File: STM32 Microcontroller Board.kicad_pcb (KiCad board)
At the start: 4 copper layers, 69.1 x 94.3 mm, 177 parts, among them J1 F407 SWD, J10 USB_B_Micro, J2 GPIO, J3 Conn_01x02_Pin, J4 F103 SWD, J5 USB_B_Micro, J6 Ethernet, J7 12V IN, J8 12V RGB LED, J9 Relay IO, Q1 PMOS, Q2 NMOS, Q3 NMOS, Q4 NMOS, SW1 SW_Push, SW2 SW_Push, SW3 SW_Push, SW4 SW_Push, SW5 SW_Push, SW6 SW_Push, U1 STM32F407VGTx, U2 MCP1825S-3302E/EB, U3 STM32F103C8T6, U4 USBLC6-2SC6, U5 DP83826IRHBR, U6 TLV9001TIDCKR, U7 ULN2803CDWR, U8 USBLC6-2SC6, Y1 8MHz, Y2 25MHz

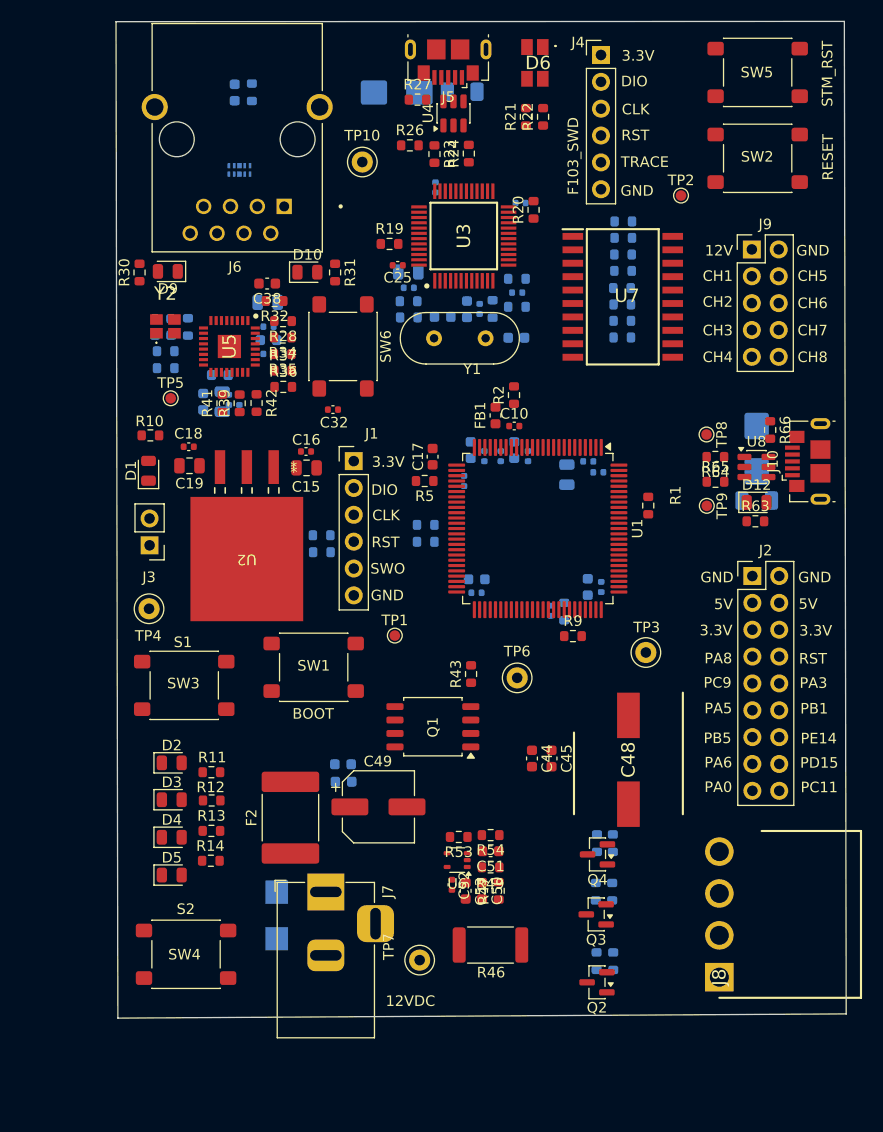
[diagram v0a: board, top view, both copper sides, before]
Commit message: Layout Routing
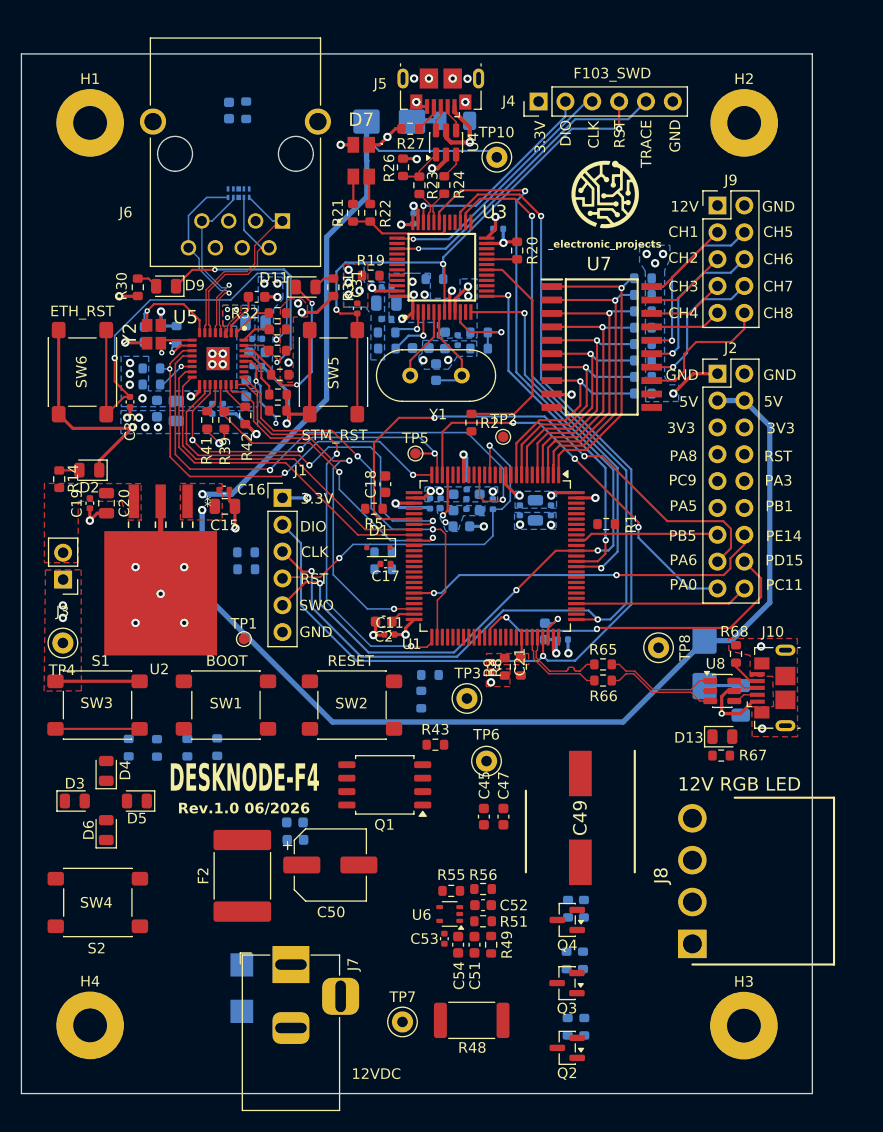
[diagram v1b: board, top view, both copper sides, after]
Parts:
- removed TP9: D-, TestPoint:TestPoint_Pad_D1.0mm
- added C17: 0.1uF, Capacitor_SMD:C_0402_1005Metric, F.Cu at (135.6, 90.7)
- added D1: 3.3V, Diode_SMD:D_SOD-323F, F.Cu at (134.9, 89.1)
- added G***: LOGO, LOGO, F.Cu at (156.3, 55.7)
- added H1: MountingHole, MountingHole:MountingHole_3.2mm_M3_Pad, F.Cu at (107.6, 48.9)
- added H2: MountingHole, MountingHole:MountingHole_3.2mm_M3_Pad, F.Cu at (169.5, 48.9)
- added H3: MountingHole, MountingHole:MountingHole_3.2mm_M3_Pad, F.Cu at (169.4, 134.3)
- added H4: MountingHole, MountingHole:MountingHole_3.2mm_M3_Pad, F.Cu at (107.6, 134.3)
- added R44: 100k, Resistor_SMD:R_0603_1608Metric, B.Cu at (138.9, 103.5)
- added R45: 22.1k, Resistor_SMD:R_0603_1608Metric, B.Cu at (139.8, 101.2)
- C10, FB1: moved to B.Cu
- C11, C2, R8: moved to F.Cu
- C21: renamed from C20; moved to F.Cu
- C26: renamed from C25; moved to B.Cu
- C31: renamed from C30; moved to F.Cu
- C6: value 0.1uF -> 1uF; footprint Capacitor_SMD:C_0402_1005Metric -> Capacitor_SMD:C_0603_1608Metric
- C7: value 1uF -> 0.1uF; footprint Capacitor_SMD:C_0603_1608Metric -> Capacitor_SMD:C_0402_1005Metric
- R10: renamed from R11; moved to B.Cu
- R11: renamed from R12; moved to B.Cu
- R12: renamed from R13; moved to B.Cu
- R13: renamed from R14; moved to B.Cu
- TP8: value D+ -> 5V; footprint TestPoint:TestPoint_Pad_D1.0mm -> TestPoint:TestPoint_Keystone_5000-5004_Miniature
- U4, U8: value USBLC6-2SC6 -> USBLC6-2
- moved SW2 64.4 mm to (132.4, 104.0)
- moved SW5 49.1 mm to (130.6, 72.5), turned to 90 degrees
- moved TP2 28.4 mm to (146.7, 78.6), turned to 90 degrees
- moved C11 24.9 mm to (135.9, 97.3), turned to 180 degrees
- moved SW6 24.8 mm to (106.9, 72.5), turned to 90 degrees
- moved TP5 23.7 mm to (138.4, 80.2)
- moved R67 22.4 mm to (167.3, 108.8)
- moved D13 22.4 mm to (167.4, 107.0)
- moved R65 22.3 mm to (156.1, 100.2)
- moved J10 21.7 mm to (172.2, 102.4)
- moved R66 21.6 mm to (156.1, 101.7)
- moved R68 21.4 mm to (168.7, 99.2)
- moved U8 21.4 mm to (167.4, 102.7)
- moved D14 20.9 mm to (165.7, 100.0)
- moved TP8 20.7 mm to (161.4, 98.6)
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- renumbered C17 to C18, C18 to C19, C19 to C20, C21 to C22, C22 to C23, C23 to C24, C24 to C25, C26 to C27, C27 to C28, C28 to C29, C29 to C30, C31 to C32, C32 to C33, C33 to C34, C34 to C35, C35 to C36, C38 to C37, C36 to C38, C37 to C39, C39 to C40, C40 to C41, C41 to C42, C42 to C43, C43 to C44, C44 to C45, C45 to C47, C47 to C48, C48 to C49, C49 to C50, C50 to C51, C51 to C52, C52 to C53, C53 to C54, D8 to D10, D10 to D11, D11 to D12, D12 to D13, D13 to D14, D1 to D2, D2 to D3, D3 to D4, D4 to D5, D5 to D6, D6 to D7, D7 to D8, R10 to R14, R44 to R46, R45 to R47, R46 to R48, R47 to R49, R48 to R50, R49 to R51, R50 to R52, R51 to R53, R52 to R54, R53 to R55, R54 to R56, R55 to R57, R56 to R58, R57 to R59, R58 to R60, R59 to R61, R60 to R62, R61 to R63, R62 to R64, R64 to R65, R65 to R66, R63 to R67, R66 to R68
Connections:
- net /Debugger/USB_DN renamed /Debugger/USB_N
- net /Debugger/USB_DP renamed /Debugger/USB_P
- net Net-(R64-Pad1) renamed /AC PWR ctrl & USB FS/USB_FS_DP
- net Net-(R65-Pad2) renamed /AC PWR ctrl & USB FS/USB_FS_DN
- C6 pad 1: +3.3V -> Net-(U1-VDDA)
- C7 pad 1: Net-(U1-VDDA) -> +3.3V
- C8 pad 1: +3.3V -> Net-(U1-VDDA)
- C9 pad 1: Net-(U1-VDDA) -> +3.3V
- D10 pad 1: /Ethernet PHY/RD_N -> /Ethernet PHY/TD_P
- D10 pad 2: /Ethernet PHY/RD_P -> /Ethernet PHY/TD_N
- D10 pad 4: /Ethernet PHY/TD_N -> /Ethernet PHY/RD_P
- D10 pad 5: /Ethernet PHY/TD_P -> /Ethernet PHY/RD_N
- D8 pad 2: Net-(D7-A) -> Net-(D8-A)
- F1 pad 1: Net-(D7-A) -> Net-(D8-A)
- J2 pad 12: /Main MCU/PB1 -> /Main MCU/PC8
- TP8 pad 1: /AC PWR ctrl & USB FS/USB_OTG_FS_DP -> +5V
- U1 pad 65: unconnected-(U1-PC8-Pad65) -> /Main MCU/PC8
- U4 pad 5: Net-(D7-A) -> Net-(J5-VBUS)
- U8 pad 5: /AC PWR ctrl & USB FS/USB_OTG_FS_VBUS -> Net-(J10-VBUS)
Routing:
- net +5V: track 0.00 -> 153.5 mm, vias 0 -> 2
- net GND: track 0.00 -> 108.0 mm, vias 0 -> 57
- net /Main MCU/T_SWDIO: track 0.00 -> 96.6 mm, vias 0 -> 2
- net /Main MCU/T_SWCLK: track 0.00 -> 92.3 mm, vias 0 -> 3
- net /Main MCU/T_SWO: track 0.00 -> 88.0 mm, vias 0 -> 4
- net /Debugger/STM_RST: track 0.00 -> 57.2 mm, vias 0 -> 3
- net +3.3V: track 0.00 -> 56.8 mm, vias 0 -> 30
- net /Main MCU/RESET: track 0.00 -> 55.9 mm, vias 0 -> 2
- net /Main MCU/PA6: track 0.00 -> 53.5 mm, vias 0 -> 2
- net /Ethernet PHY/MDC: track 0.00 -> 52.5 mm, vias 0 -> 2
- net /Ethernet PHY/PHY_RST: track 0.00 -> 46.6 mm, vias 0 -> 2
- net /Ethernet PHY/TX_D0: track 0.00 -> 40.8 mm, vias 0 -> 2
- net /Ethernet PHY/MDIO: track 0.00 -> 40.7 mm, vias 0 -> 3
- net /Ethernet PHY/CRS_DV: track 0.00 -> 38.9 mm, vias 0 -> 2
- net /Ethernet PHY/TX_D1: track 0.00 -> 38.8 mm, vias 0 -> 2
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- added copper zone on B.Cu, net +3.3V
- added copper zone on F.Cu, net +3.3V
- added copper zone on In2.Cu, net +3.3V
- added copper zone on F.Cu, net +5V
- added copper zone on F.Cu, net /Main MCU/PA9
- added copper zone on B.Cu, net GND
- added copper zone on F.Cu, net GND
- added copper zone on In1.Cu, net GND
- added copper zone on F.Cu, net Net-(J3-Pin_2)
- added copper zone on B.Cu, net Net-(U1-VDDA)
- added copper zone on B.Cu, net Net-(U5-VDDA3V3)
- added copper zone on F.Cu, net Net-(U5-VDDA3V3)
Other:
- board size 69.1 x 94.3 mm -> 74.8 x 98.3 mm
- board text added: "3V3"
- board text added: "DESKNODE-F4"
- board text added: "ETH_RST"
- board text added: "Rev.1.0 06/2026"
- board text added: "_electronic_projects"
